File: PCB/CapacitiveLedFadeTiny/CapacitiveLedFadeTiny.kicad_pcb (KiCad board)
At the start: 2 copper layers, 36.3 x 36.3 mm, 16 parts, among them J3 LEDs, J4 Antenna

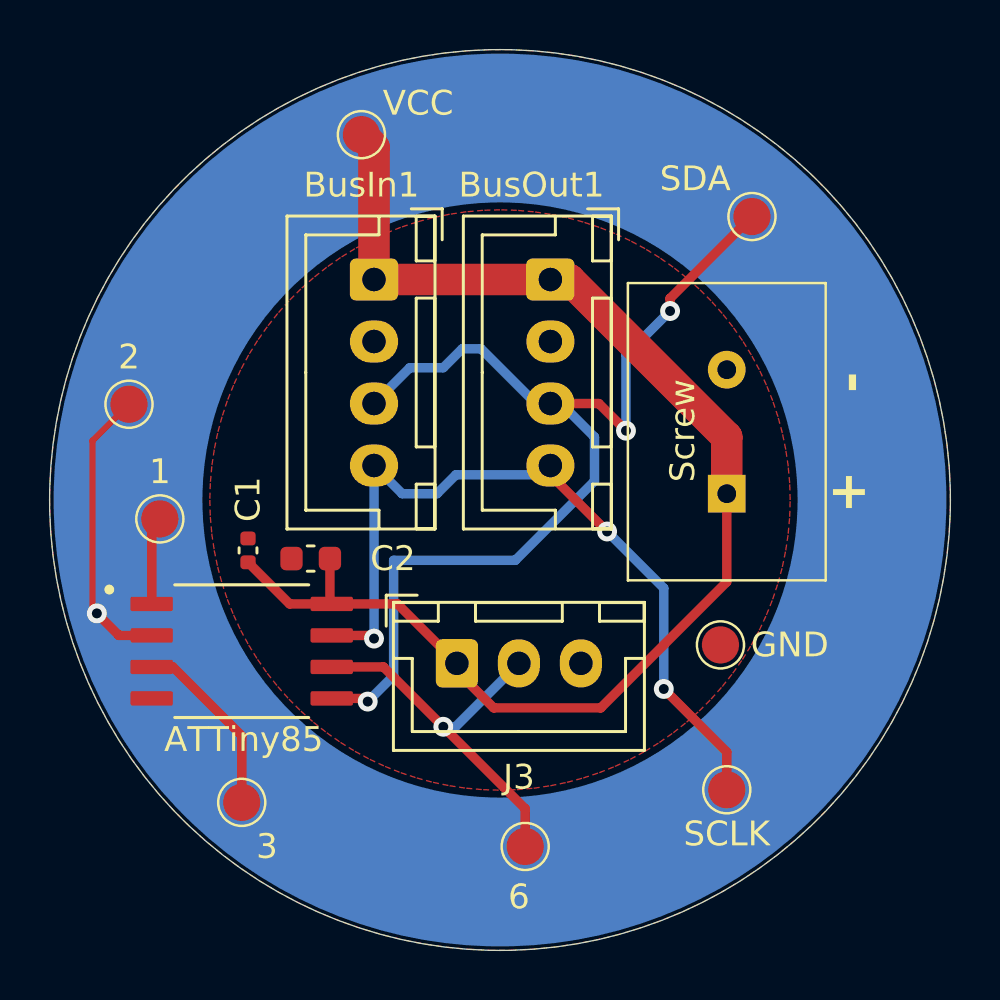
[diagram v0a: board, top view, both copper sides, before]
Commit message: v3 pcb
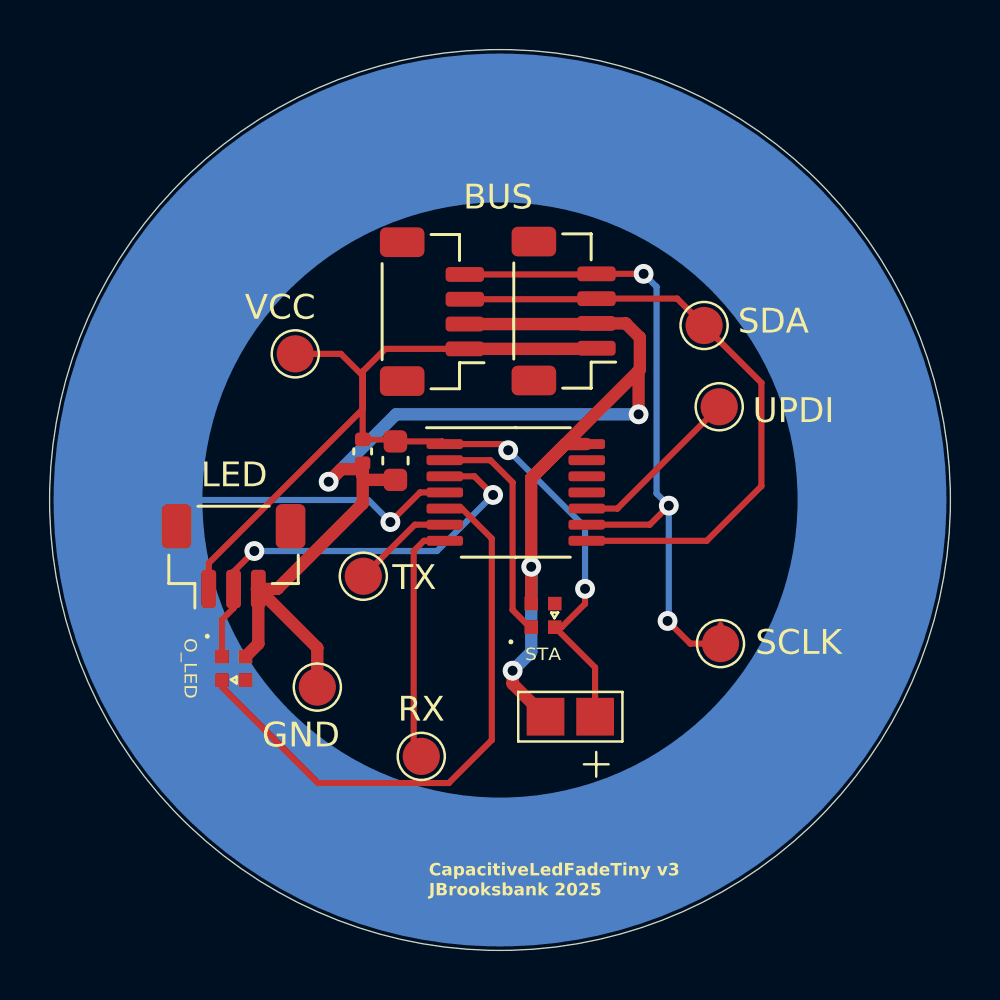
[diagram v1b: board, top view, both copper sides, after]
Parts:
- removed 1: 1, Library:TestPoint_Pad_1.5mm_circular
- removed 2: 2, Library:TestPoint_Pad_1.5mm_circular
- removed 3: 3, Library:TestPoint_Pad_1.5mm_circular
- removed 6: 6, Library:TestPoint_Pad_1.5mm_circular
- removed ATTiny85: ATTINY85-20SU, ATTINY85-20SFR:SOIC127P798X216-8N
- removed BusIn1: Bus In, Connector_JST:JST_XH_B4B-XH-A_1x04_P2.50mm_Vertical
- removed C1: 1uF, Capacitor_SMD:C_0402_1005Metric
- removed C2: 0.1uF, Capacitor_SMD:C_0603_1608Metric
- removed J3: LEDs, Connector_JST:JST_XH_B3B-XH-A_1x03_P2.50mm_Vertical
- removed J4: Antenna, TestPoint:TestPoint_Pad_1.0x1.0mm
- removed Screw: Power Inject, Library:SCREW_TERMINAL_5mm_01x02
- added BUS: Bus In, Connector_JST:JST_SH_BM04B-SRSS-TB_1x04-1MP_P1.00mm_Vertical, F.Cu at (126.3, 88.9)
- added C3: 0.1uf, Capacitor_SMD:C_0402_1005Metric, F.Cu at (123.5, 94.6)
- added C4: 1uf, Capacitor_SMD:C_0603_1608Metric, F.Cu at (124.8, 94.9)
- added J1: Antenna, CapacitiveLedFadeLibrary:CapacitiveAntenna, F.Cu at (177.1, 85.3)
- added J6: Power Inject, Library:2Pad, F.Cu at (131.9, 105.3)
- added LED: LEDs, Connector_JST:JST_SH_BM03B-SRSS-TB_1x03-1MP_P1.00mm_Vertical, F.Cu at (118.3, 98.8)
- added O_LED: ~, CapacitiveLedFadeLibrary:SK6805-EC15, F.Cu at (118.3, 103.3)
- added RX: PadRX, Library:TestPoint_Pad_1.5mm_circular, F.Cu at (125.9, 106.9)
- added STA: ~, CapacitiveLedFadeLibrary:SK6805-EC15, F.Cu at (130.8, 101.2)
- added TX: PadTX, Library:TestPoint_Pad_1.5mm_circular, F.Cu at (123.5, 99.6)
- added U1: ATtiny3224-X, Package_SO:TSSOP-14_4.4x5mm_P0.65mm, F.Cu at (129.7, 96.2)
- added UPDI: PadUPDI, Library:TestPoint_Pad_1.5mm_circular, F.Cu at (137.9, 92.8)
- BusOut1: footprint Connector_JST:JST_XH_B4B-XH-A_1x04_P2.50mm_Vertical -> Connector_JST:JST_SH_BM04B-SRSS-TB_1x04-1MP_P1.00mm_Vertical
- moved GND 16.3 mm to (121.7, 104.1)
- moved VCC 9.23 mm to (120.8, 90.6)
- moved SCLK 5.90 mm to (137.9, 102.3)
- moved SDA 4.80 mm to (137.3, 89.5)
- moved BusOut1 1.38 mm to (131.6, 88.9), turned to 90 degrees
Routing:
- net GND: track 0.00 -> 63.8 mm, vias 0 -> 4
- net Net-(LED1-VDD): track 0.00 -> 24.0 mm
- net /2: track 19.3 -> 0.00 mm, vias 1 -> 0
- net /SDA: track 44.4 -> 25.5 mm, vias 3 -> 0
- net /LED_Signal: track 0.00 -> 17.6 mm, vias 0 -> 2
- net /6: track 15.8 -> 0.00 mm, vias 1 -> 0
- net Net-(J1-Pin_1): track 0.00 -> 13.6 mm, vias 0 -> 1
- net /RX: track 0.00 -> 9.83 mm
- net Net-(LED2-DIN): track 0.00 -> 9.29 mm
- net VCC: track 54.6 -> 47.0 mm, vias 0 -> 2
- net /3: track 7.47 -> 0.00 mm
- net /UPDI: track 0.00 -> 7.04 mm
- net /SCLK: track 32.8 -> 28.5 mm
- net /TX: track 0.00 -> 4.15 mm
- net /1: track 3.56 -> 0.00 mm
- removed copper zone on F.Cu, net GND
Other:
- board text added: "CapacitiveLedFadeTiny v3 JBrooksbank 2025"
- board text removed: "+"
- board text removed: "-"
